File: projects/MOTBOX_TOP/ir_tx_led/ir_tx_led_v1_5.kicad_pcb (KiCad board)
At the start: 2 copper layers, 23 x 40 mm, 10 parts, among them J1 Conn_01x03

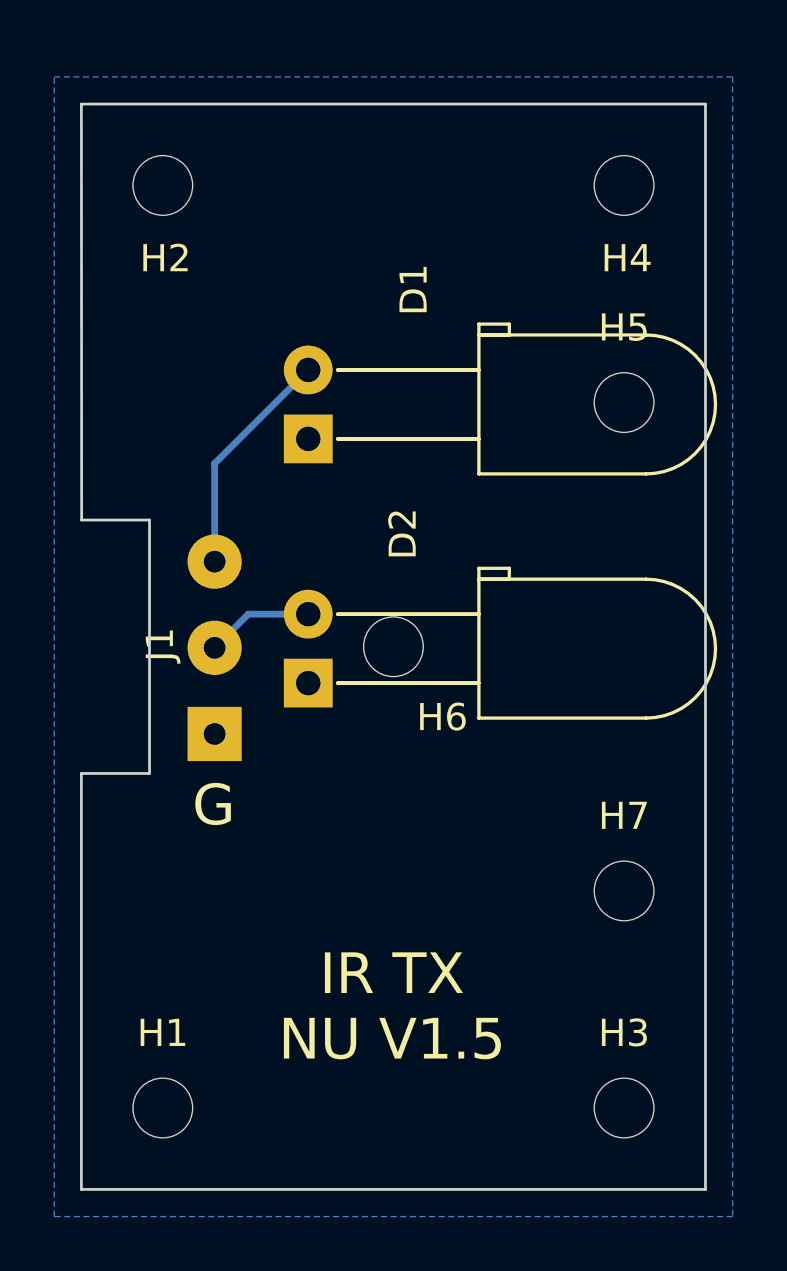
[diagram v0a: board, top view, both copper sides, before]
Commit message: Changes for improvments
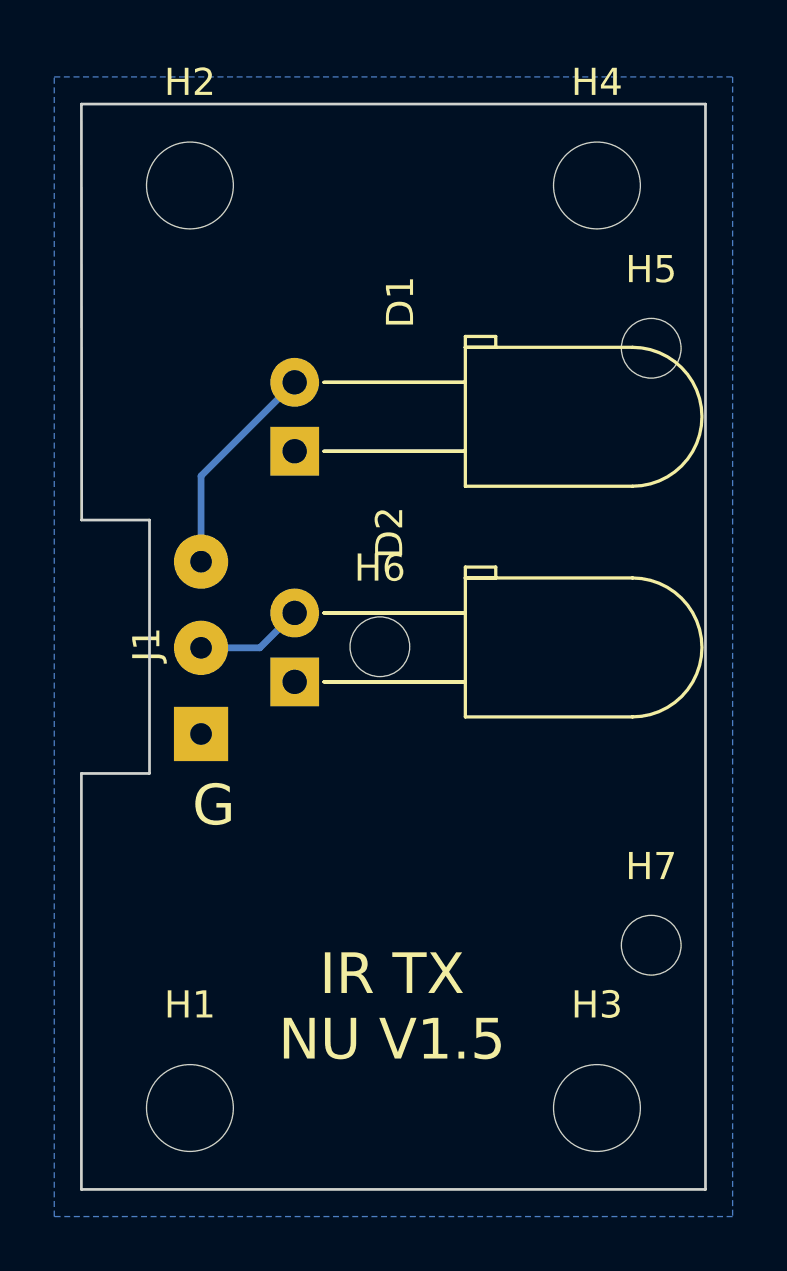
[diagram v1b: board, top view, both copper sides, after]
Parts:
- H1, H2, H3, H4: footprint MountingHole:MountingHole_2.2mm_M2_ISO7380 -> MountingHole:MountingHole_3.2mm_M3_DIN965
- H5, H6, H7: footprint MountingHole:MountingHole_2.2mm_M2_ISO7380 -> MountingHole:MountingHole_2.2mm_M2_DIN965
- moved H5 2.24 mm to (138.3, 81.5)
- moved H7 2.24 mm to (138.3, 103.5)
- moved H1 1.00 mm to (121.3, 109.5)
- moved H2 1.00 mm to (121.3, 75.5)
- moved H3 1.00 mm to (136.3, 109.5)
- moved H4 1.00 mm to (136.3, 75.5)
- moved D1 0.68 mm to (125.2, 85.3)
- moved D2 0.50 mm to (125.2, 93.8)
- moved H6 0.50 mm to (128.3, 92.5)
- moved J1 0.50 mm to (121.7, 95.7)
